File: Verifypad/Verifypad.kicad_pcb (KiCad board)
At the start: 2 copper layers, 46 x 42.5 mm, 4 parts, among them SW1 SW_Push, SW2 SW_Push, U1 MOUDLE-SEEEDUINO-XIAO

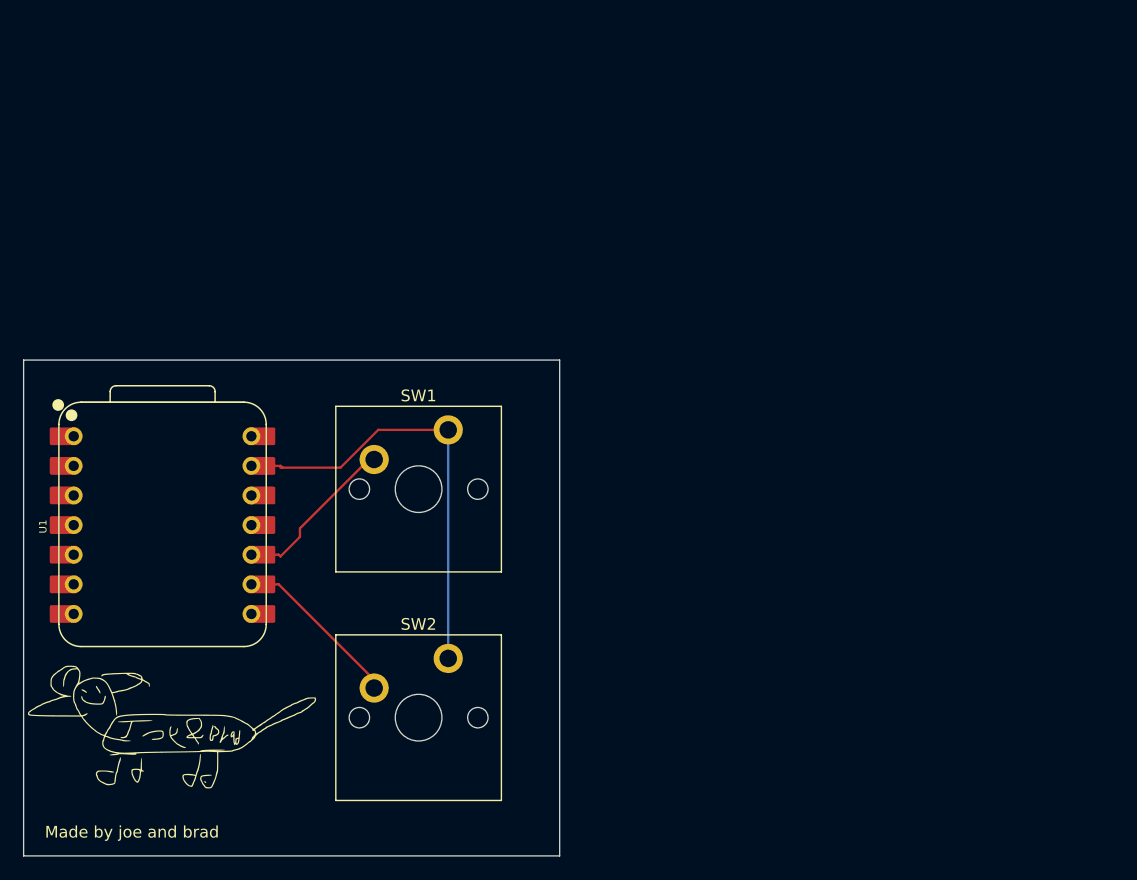
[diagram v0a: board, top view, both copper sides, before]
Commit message: Kicad
new kicad stuff :)
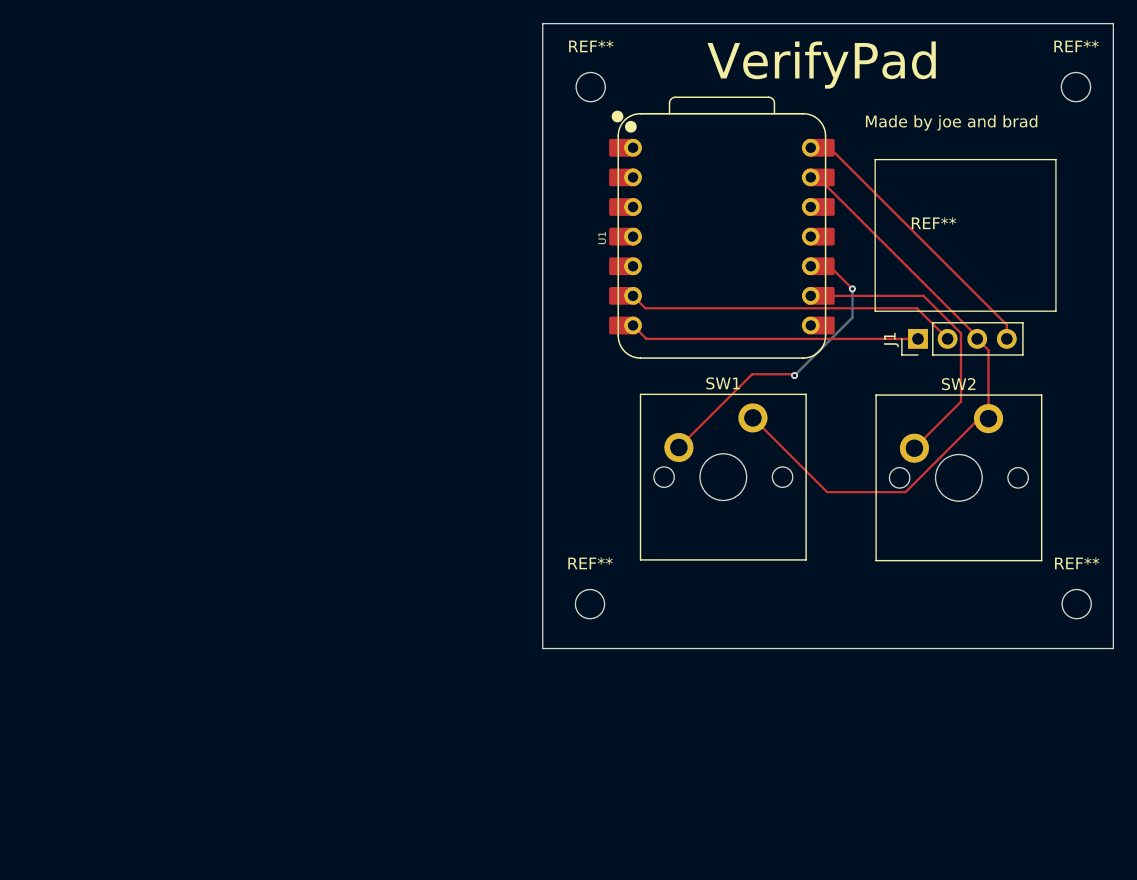
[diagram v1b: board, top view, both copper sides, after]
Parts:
- added J1: Conn_01x04, Connector_PinHeader_2.54mm:PinHeader_1x04_P2.54mm_Vertical, F.Cu at (192.3, 72.6)
- added REF**: MountingHole_2.5mm, MountingHole:MountingHole_2.5mm, F.Cu at (164.2, 51.0)
- added REF**: MountingHole_2.5mm, MountingHole:MountingHole_2.5mm, F.Cu at (164.2, 95.3)
- added REF**: MountingHole_2.5mm, MountingHole:MountingHole_2.5mm, F.Cu at (205.8, 51.0)
- added REF**: 0.49Display, Verifypad:0.49Display, F.Cu at (193.6, 63.2)
- added REF**: MountingHole_2.5mm, MountingHole:MountingHole_2.5mm, F.Cu at (205.9, 95.3)
- G***: moved to B.Cu
- moved U1 54.0 mm to (175.5, 63.8)
- moved SW2 50.7 mm to (195.8, 84.5)
- moved G*** 48.6 mm to (175.7, 92.2), turned to 180 degrees
- moved SW1 26.1 mm to (175.6, 84.4)
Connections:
- U1 pad 14: unconnected-(U1-5V-Pad14)_1 -> /VCC
- U1 pad 6: unconnected-(U1-PA9_A5_D5_SCL-Pad6)_1 -> /I2CD
- U1 pad 7: unconnected-(U1-PB08_A6_D6_TX-Pad7)_1 -> /I2CC
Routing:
- net /I2CD: track 0.00 -> 28.5 mm
- net /I2CC: track 0.00 -> 24.9 mm
- net /VCC: track 0.00 -> 24.3 mm
- net GND: track 38.1 -> 52.8 mm
- net Net-(U1-PA5_A9_D9_MISO): track 14.5 -> 26.4 mm, vias 0 -> 2
- net Net-(U1-PA7_A8_D8_SCK): track 14.6 -> 25.7 mm
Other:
- board size 46 x 42.5 mm -> 48.9 x 53.6 mm
- board text added: "VerifyPad"
